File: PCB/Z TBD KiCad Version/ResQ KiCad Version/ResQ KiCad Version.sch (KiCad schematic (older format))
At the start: 7 parts

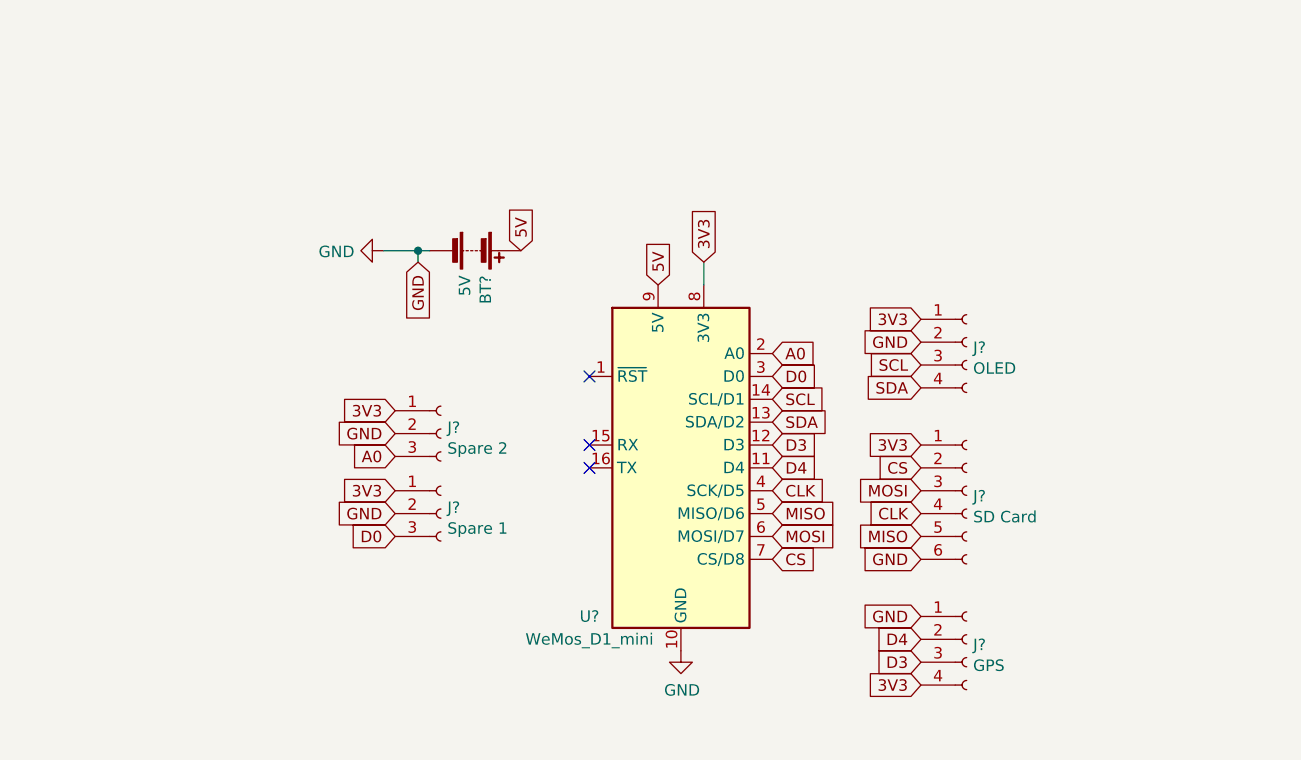
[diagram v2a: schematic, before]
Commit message: Updated Kicad Schem
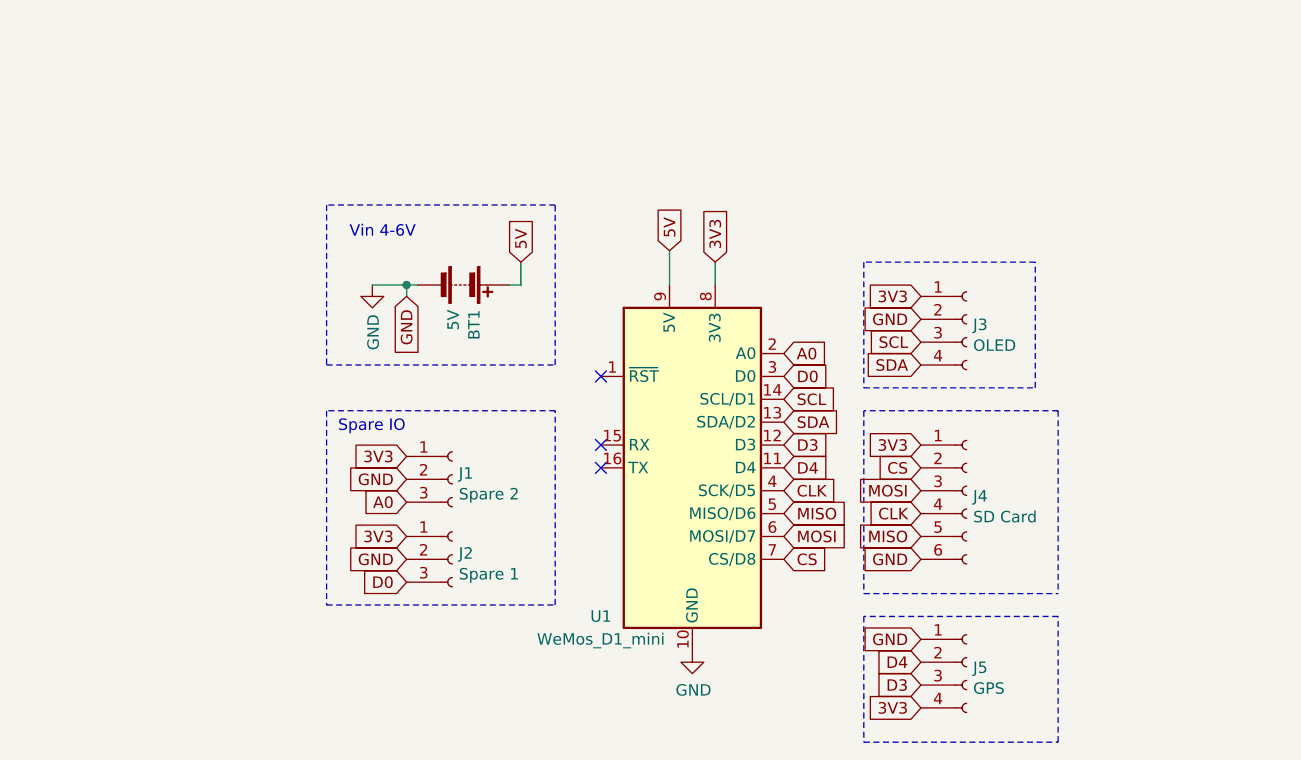
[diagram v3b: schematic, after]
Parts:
- gave numbers to parts that had none: 7
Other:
- note added: "Spare IO"
- note added: "Vin 4-6V"
- moved on the sheet: BT1, J1, J2, J3, J5, U1
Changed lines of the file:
@@
 $EndDescr
 $Comp
-L Connector:Conn_01x06_Female J?
+L Connector:Conn_01x06_Female J4
 U 1 1 5F31DE3A
 P 9050 5400
-F 0 "J?" H 9078 5376 50  0000 L CNN
+F 0 "J4" H 9078 5376 50  0000 L CNN
 F 1 "SD Card" H 9078 5285 50  0000 L CNN
 F 2 "" H 9050 5400 50  0001 C CNN
@@
 Text GLabel 8850 5500 0    50   Input ~ 0
 CLK
-Text GLabel 8200 5100 2    50   Input ~ 0
+Text GLabel 8850 5200 0    50   Input ~ 0
+3V3
+Text GLabel 8850 5700 0    50   Input ~ 0
+GND
+Text GLabel 8250 5700 2    50   Input ~ 0
+CS
+Text GLabel 8250 5600 2    50   Input ~ 0
+MOSI
+Text GLabel 8250 5500 2    50   Input ~ 0
+MISO
+Text GLabel 8250 5400 2    50   Input ~ 0
+CLK
+Text GLabel 7950 4400 1    50   Input ~ 0
+3V3
+Text GLabel 8850 6050 0    50   Input ~ 0
+GND
+Text GLabel 8850 6350 0    50   Input ~ 0
+3V3
+Text GLabel 8850 6150 0    50   Input ~ 0
+D4
+Text GLabel 8250 5300 2    50   Input ~ 0
+D4
+Text GLabel 8250 5200 2    50   Input ~ 0
+D3
+Text GLabel 8850 6250 0    50   Input ~ 0
+D3
+$Comp
+L power:GND #PWR02
+U 1 1 5F34FDAC
+P 7850 6100
+F 0 "#PWR02" H 7850 5850 50  0001 C CNN
+F 1 "GND" H 7855 5927 50  0000 C CNN
+F 2 "" H 7850 6100 50  0001 C CNN
+F 3 "" H 7850 6100 50  0001 C CNN
+	1    7850 6100
+	1    0    0    -1
+$EndComp
+$Comp
+L Connector:Conn_01x04_Female J5
+U 1 1 5F321884
+P 9050 6150
+F 0 "J5" H 9078 6126 50  0000 L CNN
+F 1 "GPS" H 9078 6035 50  0000 L CNN
+F 2 "" H 9050 6150 50  0001 C CNN
+F 3 "~" H 9050 6150 50  0001 C CNN
+	1    9050 6150
+	1    0    0    -1
+$EndComp
+NoConn ~ 7450 4900
+NoConn ~ 7450 5200
+NoConn ~ 7450 5300
+Wire Wire Line
+	7950 4400 7950 4500
+$Comp
+L Connector:Conn_01x03_Female J2
+U 1 1 5F322635
+P 6800 5700
+F 0 "J2" H 6828 5726 50  0000 L CNN
+F 1 "Spare 1" H 6828 5635 50  0000 L CNN
+F 2 "" H 6800 5700 50  0001 C CNN
+F 3 "~" H 6800 5700 50  0001 C CNN
+	1    6800 5700
+	1    0    0    -1
+$EndComp
+Text GLabel 6600 5800 0    50   Input ~ 0
+D0
+Text GLabel 6600 5700 0    50   Input ~ 0
+GND
+$Comp
+L Connector:Conn_01x03_Female J1
+U 1 1 5F3230C4
+P 6800 5350
+F 0 "J1" H 6828 5376 50  0000 L CNN
+F 1 "Spare 2" H 6828 5285 50  0000 L CNN
+F 2 "" H 6800 5350 50  0001 C CNN
+F 3 "~" H 6800 5350 50  0001 C CNN
+	1    6800 5350
+	1    0    0    -1
+$EndComp
+Text GLabel 6600 5250 0    50   Input ~ 0
+3V3
+Text GLabel 6600 5350 0    50   Input ~ 0
+GND
+Text GLabel 6600 5600 0    50   Input ~ 0
+3V3
+Text GLabel 6600 5450 0    50   Input ~ 0
+A0
+Wire Wire Line
+	6650 4500 6600 4500
+Text GLabel 6600 4550 3    50   Input ~ 0
+GND
+$Comp
+L power:GND #PWR01
+U 1 1 5F34EF30
+P 6450 4500
+F 0 "#PWR01" H 6450 4250 50  0001 C CNN
+F 1 "GND" V 6455 4372 50  0000 R CNN
+F 2 "" H 6450 4500 50  0001 C CNN
+F 3 "" H 6450 4500 50  0001 C CNN
+	1    6450 4500
+	1    0    0    -1
+$EndComp
+$Comp
+L Device:Battery BT1
+U 1 1 5F31A8A9
+P 6850 4500
+F 0 "BT1" H 6958 4546 50  0000 L CNN
+F 1 "5V" H 6958 4455 50  0000 L CNN
+F 2 "" V 6850 4560 50  0001 C CNN
+F 3 "~" V 6850 4560 50  0001 C CNN
+	1    6850 4500
+	0    1    1    0
+$EndComp
+Text GLabel 7750 4350 1    50   Input ~ 0
+5V
+$Comp
+L MCU_Module:WeMos_D1_mini U1
+U 1 1 5F31691B
+P 7850 5300
+F 0 "U1" H 7450 4650 50  0000 C CNN
+F 1 "WeMos_D1_mini" H 7450 4550 50  0000 C CNN
+F 2 "Module:WEMOS_D1_mini_light" H 7850 4150 50  0001 C CNN
+F 3 "https://wiki.wemos.cc/products:d1:d1_mini#documentation" H 6000 4150 50  0001 C CNN
+	1    7850 5300
+	1    0    0    -1
+$EndComp
+Text GLabel 7100 4400 1    50   Input ~ 0
+5V
+Wire Wire Line
+	6600 4500 6600 4550
+Text Notes 6350 4300 0    50   ~ 0
+Vin 4-6V
+Wire Wire Line
+	7100 4400 7100 4500
+Wire Wire Line
+	7100 4500 7050 4500
+Connection ~ 6600 4500
+Wire Wire Line
+	6450 4500 6600 4500
+Wire Notes Line
+	6250 4150 6250 4850
+Wire Notes Line
+	6250 4850 7250 4850
+Wire Notes Line
+	7250 4850 7250 4150
+Wire Notes Line
+	7250 4150 6250 4150
+Text GLabel 8250 5100 2    50   Input ~ 0
 SDA
-Text GLabel 8200 5000 2    50   Input ~ 0
+Wire Notes Line
+	6250 5050 6250 5900
+Wire Notes Line
+	6250 5900 7250 5900
+Wire Notes Line
+	7250 5900 7250 5050
+Wire Notes Line
+	7250 5050 6250 5050
+Text Notes 6300 5150 0    50   ~ 0
+Spare IO
+Wire Notes Line
+	8600 5850 9450 5850
+Wire Notes Line
+	9450 5050 8600 5050
+Wire Notes Line
+	8600 5950 8600 6500
+Wire Notes Line
+	8600 6500 9450 6500
+Wire Notes Line
+	9450 6500 9450 5950
+Wire Notes Line
+	9450 5950 8600 5950
+Wire Notes Line
+	8600 4400 8600 4950
+Wire Notes Line
+	9350 4400 8600 4400
+Wire Notes Line
+	9350 4950 9350 4400
+Wire Notes Line
+	8600 4950 9350 4950
+Text GLabel 8250 5000 2    50   Input ~ 0
 SCL
-Text GLabel 8850 5200 0    50   Input ~ 0
-3V3
-Text GLabel 8850 5700 0    50   Input ~ 0
-GND
-Text GLabel 8200 4900 2    50   Input ~ 0
+Text GLabel 8850 4850 0    50   Input ~ 0
+SDA
+Text GLabel 8850 4750 0    50   Input ~ 0
+SCL
+Text GLabel 8850 4550 0    50   Input ~ 0
+3V3
+Text GLabel 8850 4650 0    50   Input ~ 0
+GND
+$Comp
+L Connector:Conn_01x04_Female J3
+U 1 1 5F31F299
+P 9050 4650
+F 0 "J3" H 9078 4626 50  0000 L CNN
+F 1 "OLED" H 9078 4535 50  0000 L CNN
+F 2 "" H 9050 4650 50  0001 C CNN
+F 3 "~" H 9050 4650 50  0001 C CNN
+	1    9050 4650
+	1    0    0    -1
+$EndComp
+Text GLabel 8250 4800 2    50   Input ~ 0
+A0
+Text GLabel 8250 4900 2    50   Input ~ 0
 D0
-Text GLabel 8200 4800 2    50   Input ~ 0
-A0
-Text GLabel 8200 5700 2    50   Input ~ 0
-CS
-Text GLabel 8200 5600 2    50   Input ~ 0
-MOSI
-Text GLabel 8200 5500 2    50   Input ~ 0
-MISO
-Text GLabel 8200 5400 2    50   Input ~ 0
-CLK
-Text GLabel 8850 4950 0    50   Input ~ 0
-SDA
-Text GLabel 8850 4850 0    50   Input ~ 0
-SCL
-Text GLabel 7900 4400 1    50   Input ~ 0
-3V3
-Text GLabel 8850 5950 0    50   Input ~ 0
-GND
-Text GLabel 8850 6250 0    50   Input ~ 0
-3V3
-Text GLabel 8850 4650 0    50   Input ~ 0
-3V3
-Text GLabel 8850 4750 0    50   Input ~ 0
-GND
-Text GLabel 8850 6050 0    50   Input ~ 0
-D4
-Text GLabel 8200 5300 2    50   Input ~ 0
-D4
-Text GLabel 8200 5200 2    50   Input ~ 0
-D3
-Text GLabel 8850 6150 0    50   Input ~ 0
-D3
-$Comp
-L power:GND #PWR?
-U 1 1 5F34FDAC
-P 7800 6100
-F 0 "#PWR?" H 7800 5850 50  0001 C CNN
-F 1 "GND" H 7805 5927 50  0000 C CNN
-F 2 "" H 7800 6100 50  0001 C CNN
-F 3 "" H 7800 6100 50  0001 C CNN
-	1    7800 6100
-	1    0    0    -1
-$EndComp
-$Comp
-L Connector:Conn_01x04_Female J?
-U 1 1 5F31F299
-P 9050 4750
-F 0 "J?" H 9078 4726 50  0000 L CNN
-F 1 "OLED" H 9078 4635 50  0000 L CNN
-F 2 "" H 9050 4750 50  0001 C CNN
-F 3 "~" H 9050 4750 50  0001 C CNN
-	1    9050 4750
-	1    0    0    -1
-$EndComp
-$Comp
-L Connector:Conn_01x04_Female J?
-U 1 1 5F321884
-P 9050 6050
-F 0 "J?" H 9078 6026 50  0000 L CNN
-F 1 "GPS" H 9078 5935 50  0000 L CNN
-F 2 "" H 9050 6050 50  0001 C CNN
-F 3 "~" H 9050 6050 50  0001 C CNN
-	1    9050 6050
-	1    0    0    -1
-$EndComp
-NoConn ~ 7400 4900
-NoConn ~ 7400 5200
-NoConn ~ 7400 5300
-Wire Wire Line
-	7900 4400 7900 4500
-$Comp
-L Connector:Conn_01x03_Female J?
-U 1 1 5F322635
-P 6750 5500
-F 0 "J?" H 6778 5526 50  0000 L CNN
-F 1 "Spare 1" H 6778 5435 50  0000 L CNN
-F 2 "" H 6750 5500 50  0001 C CNN
-F 3 "~" H 6750 5500 50  0001 C CNN
-	1    6750 5500
-	1    0    0    -1
-$EndComp
-Text GLabel 6550 5600 0    50   Input ~ 0
-D0
-Text GLabel 6550 5500 0    50   Input ~ 0
-GND
-$Comp
-L Connector:Conn_01x03_Female J?
-U 1 1 5F3230C4
-P 6750 5150
-F 0 "J?" H 6778 5176 50  0000 L CNN
-F 1 "Spare 2" H 6778 5085 50  0000 L CNN
-F 2 "" H 6750 5150 50  0001 C CNN
-F 3 "~" H 6750 5150 50  0001 C CNN
-	1    6750 5150
-	1    0    0    -1
-$EndComp
-Text GLabel 6550 5050 0    50   Input ~ 0
-3V3
-Text GLabel 6550 5150 0    50   Input ~ 0
-GND
-Text GLabel 6550 5400 0    50   Input ~ 0
-3V3
-Text GLabel 6550 5250 0    50   Input ~ 0
-A0
-Wire Wire Line
-	6700 4350 6650 4350
-Text GLabel 6650 4400 3    50   Input ~ 0
-GND
-$Comp
-L power:GND #PWR?
-U 1 1 5F34EF30
-P 6500 4350
-F 0 "#PWR?" H 6500 4100 50  0001 C CNN
-F 1 "GND" V 6505 4222 50  0000 R CNN
-F 2 "" H 6500 4350 50  0001 C CNN
-F 3 "" H 6500 4350 50  0001 C CNN
-	1    6500 4350
-	0    1    1    0
-$EndComp
-$Comp
-L Device:Battery BT?
-U 1 1 5F31A8A9
-P 6900 4350
-F 0 "BT?" H 7008 4396 50  0000 L CNN
-F 1 "5V" H 7008 4305 50  0000 L CNN
-F 2 "" V 6900 4410 50  0001 C CNN
-F 3 "~" V 6900 4410 50  0001 C CNN
-	1    6900 4350
-	0    1    1    0
-$EndComp
-Text GLabel 7700 4500 1    50   Input ~ 0
-5V
-$Comp
-L MCU_Module:WeMos_D1_mini U?
-U 1 1 5F31691B
-P 7800 5300
-F 0 "U?" H 7400 4650 50  0000 C CNN
-F 1 "WeMos_D1_mini" H 7400 4550 50  0000 C CNN
-F 2 "Module:WEMOS_D1_mini_light" H 7800 4150 50  0001 C CNN
-F 3 "https://wiki.wemos.cc/products:d1:d1_mini#documentation" H 5950 4150 50  0001 C CNN
-	1    7800 5300
-	1    0    0    -1
-$EndComp
-Text GLabel 7100 4350 1    50   Input ~ 0
-5V
-Wire Wire Line
-	6650 4350 6650 4400
-Connection ~ 6650 4350
-Wire Wire Line
-	6650 4350 6500 4350
+Wire Notes Line
+	9450 5050 9450 5850
+Wire Notes Line
+	8600 5050 8600 5850
+Wire Wire Line
+	7750 4350 7750 4500
 $EndSCHEMATC
